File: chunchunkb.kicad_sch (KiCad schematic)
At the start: 124 parts, among them J1 BATT, J2 OLED, SW1 SW_Push, SW10 SW_Push, SW11 SW_Push, SW12 SW_Push, SW13 SW_Push, SW14 SW_Push, SW15 SW_Push, SW16 SW_Push, SW17 SW_Push, SW18 SW_Push, SW19 SW_Push, SW2 SW_Push, SW20 SW_Push, SW21 SW_Push, SW22 SW_Push, SW23 SW_Push, SW24 SW_Push, SW25 SW_Push, SW26 SW_Push, SW27 SW_Push, SW28 SW_Push, SW29 SW_Push, SW3 SW_Push, SW30 SW_Push, SW31 EC11, SW32 SW_Push, SW33 SW_Push, SW34 SW_Push, SW35 SW_Push, SW36 SW_Push, SW4 SW_Push, SW5 SW_Push, SW6 SW_Push, SW7 SW_Push, SW8 SW_Push, SW9 SW_Push

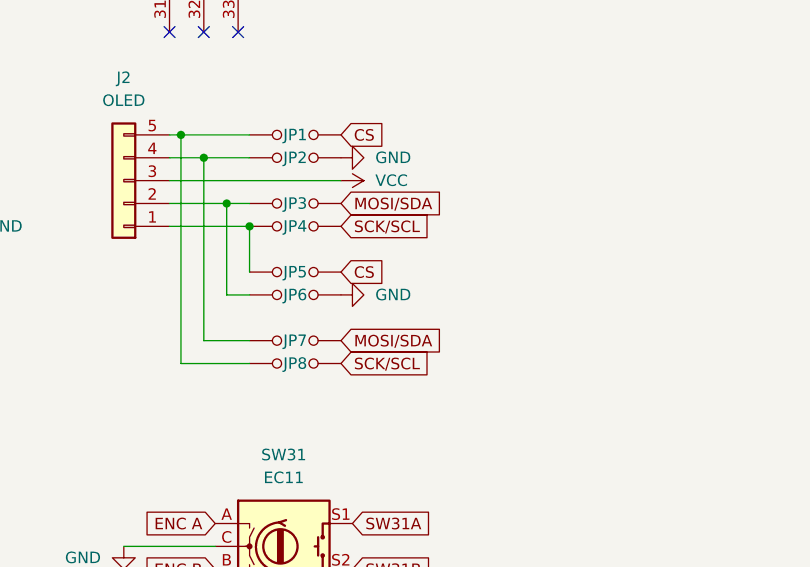
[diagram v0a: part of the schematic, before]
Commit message: snapshot
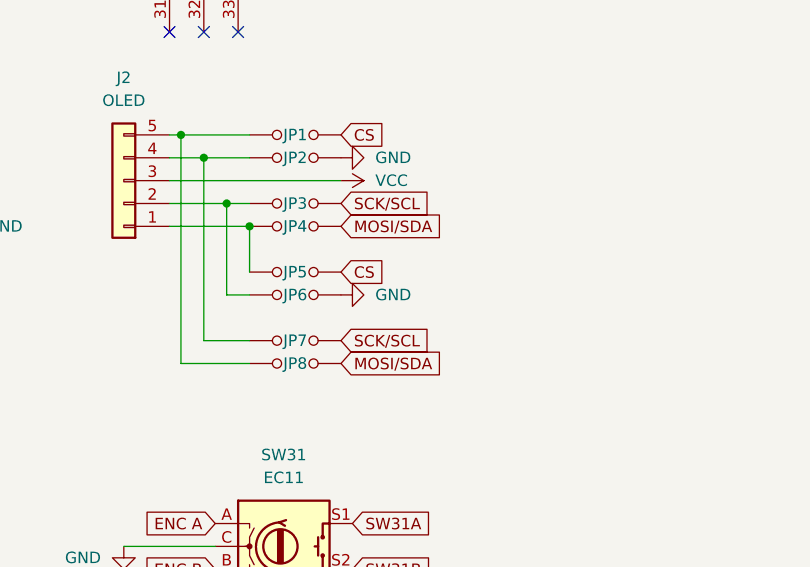
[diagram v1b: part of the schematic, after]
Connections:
- net MOSI/SDA: now also JP4.2 (B), JP8.2 (B); no longer JP3.2 (B), JP7.2 (B)
- net SCK/SCL: now also JP3.2 (B), JP7.2 (B); no longer JP4.2 (B), JP8.2 (B)

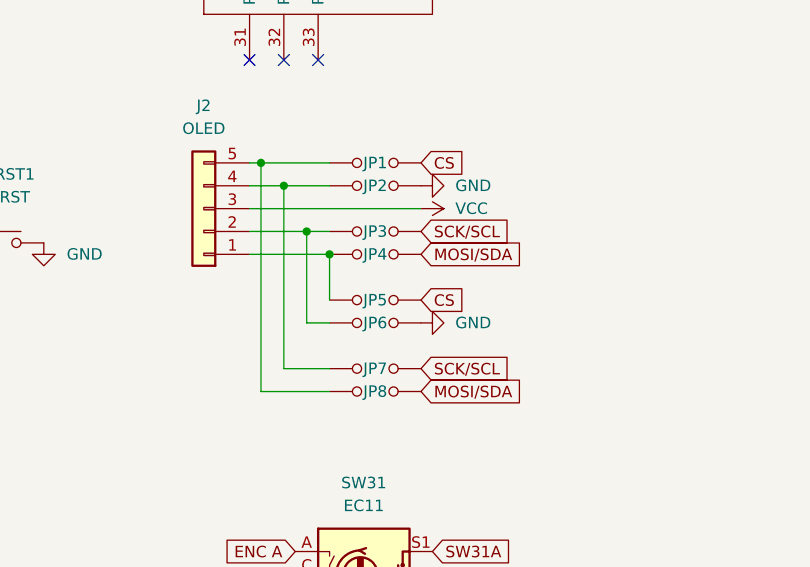
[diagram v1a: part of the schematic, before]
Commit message: snapshot
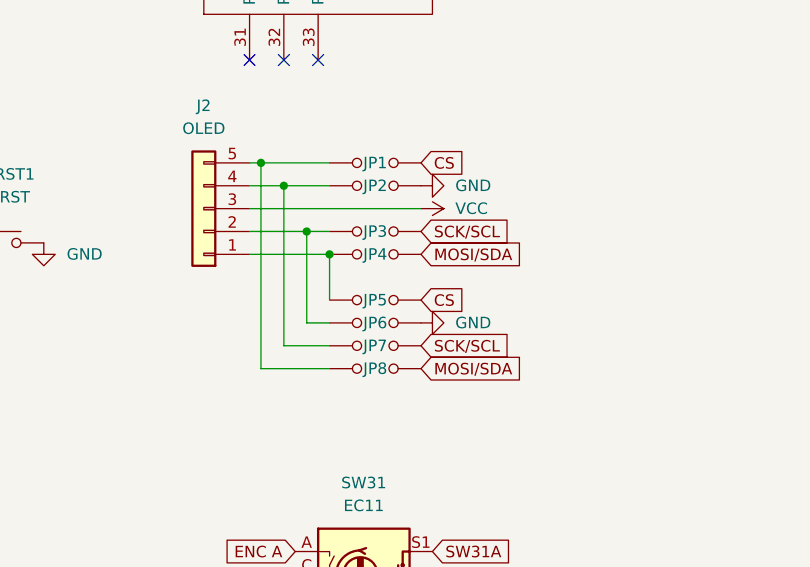
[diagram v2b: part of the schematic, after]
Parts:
- D1, D10, D11, D12, D13, D14, D15, D16, D17, D18, D19, D2, D20, D21, D22, D23, D24, D25, D26, D27, D28, D29, D3, D30, D31, D32, D33, D34, D35, D36, D4, D5, D6, D7, D8, D9: footprint chunchunkb:D_SOD-123 -> chunchunkb:crkbd-diode
- U1: footprint chunchunkb:ProMicro_R2 -> chunchunkb:ProMicro DUAL
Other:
- moved on the sheet: JP7, JP8
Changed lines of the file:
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@@
 	(wire
 		(pts
-			(xy 77.47 113.03) (xy 72.39 113.03)
+			(xy 77.47 110.49) (xy 72.39 110.49)
 		)
 		(stroke
@@
 	(wire
 		(pts
-			(xy 77.47 115.57) (xy 69.85 115.57)
+			(xy 77.47 113.03) (xy 69.85 113.03)
 		)
 		(stroke
@@
 	(wire
 		(pts
-			(xy 69.85 115.57) (xy 69.85 90.17)
+			(xy 69.85 113.03) (xy 69.85 90.17)
 		)
 		(stroke
@@
 	(wire
 		(pts
-			(xy 72.39 113.03) (xy 72.39 92.71)
+			(xy 72.39 110.49) (xy 72.39 92.71)
 		)
 		(stroke
@@
 	(global_label "SCK{slash}SCL"
 		(shape input)
-		(at 87.63 113.03 0)
+		(at 87.63 110.49 0)
 		(fields_autoplaced yes)
 		(effects
@@
 		)
 		(property "Intersheetrefs" "${INTERSHEET_REFS}"
-			(at 97.8534 113.03 0)
+			(at 97.8534 110.49 0)
 			(hide yes)
 			(show_name no)
@@
 	(global_label "MOSI{slash}SDA"
 		(shape input)
-		(at 87.63 115.57 0)
+		(at 87.63 113.03 0)
 		(fields_autoplaced yes)
 		(effects
@@
 		)
 		(property "Intersheetrefs" "${INTERSHEET_REFS}"
-			(at 98.9192 115.57 0)
+			(at 98.9192 113.03 0)
 			(hide yes)
 			(show_name no)
@@
 			)
 		)
-		(property "Footprint" "chunchunkb:D_SOD-123"
+		(property "Footprint" "chunchunkb:crkbd-diode"
 			(at 175.895 83.82 0)
 			(hide yes)
@@
 			)
 		)
-		(property "Footprint" "chunchunkb:D_SOD-123"
+		(property "Footprint" "chunchunkb:crkbd-diode"
 			(at 161.925 119.38 0)
 			(hide yes)
@@
 			)
 		)
-		(property "Footprint" "chunchunkb:D_SOD-123"
+		(property "Footprint" "chunchunkb:crkbd-diode"
 			(at 203.835 66.04 0)
 			(hide yes)
@@
 			)
 		)
-		(property "Footprint" "chunchunkb:D_SOD-123"
+		(property "Footprint" "chunchunkb:crkbd-diode"
 			(at 189.865 119.38 0)
 			(hide yes)
@@
 			)
 		)
-		(property "Footprint" "chunchunkb:D_SOD-123"
+		(property "Footprint" "chunchunkb:crkbd-diode"
 			(at 175.895 66.04 0)
 			(hide yes)
@@
 	(symbol
 		(lib_id "chunchunkb:jumper")
-		(at 82.55 115.57 0)
+		(at 82.55 113.03 0)
 		(unit 1)
 		(body_style 1)
@@
 		(fields_autoplaced yes)
 		(property "Reference" "JP8"
-			(at 82.55 115.57 0)
+			(at 82.55 113.03 0)
 			(show_name no)
 			(do_not_autoplace yes)
@@
 		)
 		(property "Value" "jumper"
-			(at 82.55 117.856 0)
+			(at 82.55 115.316 0)
 			(hide yes)
 			(show_name no)
@@
 		)
 		(property "Footprint" "chunchunkb:Jumper"
-			(at 82.55 115.57 0)
+			(at 82.55 113.03 0)
 			(hide yes)
 			(show_name no)
@@
 		)
 		(property "Datasheet" ""
-			(at 82.55 115.57 0)
+			(at 82.55 113.03 0)
 			(hide yes)
 			(show_name no)
@@
 		)
 		(property "Description" "Jumper, 2-pole, open"
-			(at 82.55 115.57 0)
+			(at 82.55 113.03 0)
 			(hide yes)
 			(show_name no)
@@
 			)
 		)
-		(property "Footprint" "chunchunkb:D_SOD-123"
+		(property "Footprint" "chunchunkb:crkbd-diode"
 			(at 217.805 83.82 0)
 			(hide yes)
@@
 			)
 		)
-		(property "Footprint" "chunchunkb:D_SOD-123"
+		(property "Footprint" "chunchunkb:crkbd-diode"
 			(at 231.775 48.26 0)
 			(hide yes)
@@
 			)
 		)
-		(property "Footprint" "chunchunkb:D_SOD-123"
+		(property "Footprint" "chunchunkb:crkbd-diode"
 			(at 203.835 83.82 0)
 			(hide yes)
@@
 			)
 		)
-		(property "Footprint" "chunchunkb:D_SOD-123"
+		(property "Footprint" "chunchunkb:crkbd-diode"
 			(at 175.895 119.38 0)
 			(hide yes)
@@
 			)
 		)
-		(property "Footprint" "chunchunkb:D_SOD-123"
+		(property "Footprint" "chunchunkb:crkbd-diode"
 			(at 231.775 101.6 0)
 			(hide yes)
@@
 			)
 		)
-		(property "Footprint" "chunchunkb:D_SOD-123"
+		(property "Footprint" "chunchunkb:crkbd-diode"
 			(at 217.805 137.16 0)
 			(hide yes)
@@
 			)
 		)
-		(property "Footprint" "chunchunkb:D_SOD-123"
+		(property "Footprint" "chunchunkb:crkbd-diode"
 			(at 231.775 66.04 0)
 			(hide yes)
@@
 			)
 		)
-		(property "Footprint" "chunchunkb:D_SOD-123"
+		(property "Footprint" "chunchunkb:crkbd-diode"
 			(at 217.805 48.26 0)
 			(hide yes)
@@
 			)
 		)
-		(property "Footprint" "chunchunkb:D_SOD-123"
+		(property "Footprint" "chunchunkb:crkbd-diode"
 			(at 161.925 101.6 0)
 			(hide yes)
@@
 			)
 		)
-		(property "Footprint" "chunchunkb:D_SOD-123"
+		(property "Footprint" "chunchunkb:crkbd-diode"
 			(at 189.865 101.6 0)
 			(hide yes)
@@
 			)
 		)
-		(property "Footprint" "chunchunkb:D_SOD-123"
+		(property "Footprint" "chunchunkb:crkbd-diode"
 			(at 161.925 83.82 0)
 			(hide yes)
@@
 			)
 		)
-		(property "Footprint" "chunchunkb:D_SOD-123"
+		(property "Footprint" "chunchunkb:crkbd-diode"
 			(at 203.835 119.38 0)
 			(hide yes)
@@
 			)
 		)
-		(property "Footprint" "chunchunkb:D_SOD-123"
+		(property "Footprint" "chunchunkb:crkbd-diode"
 			(at 217.805 101.6 0)
 			(hide yes)
@@
 			)
 		)
-		(property "Footprint" "chunchunkb:D_SOD-123"
+		(property "Footprint" "chunchunkb:crkbd-diode"
 			(at 175.895 101.6 0)
 			(hide yes)
@@
 			)
 		)
-		(property "Footprint" "chunchunkb:D_SOD-123"
+		(property "Footprint" "chunchunkb:crkbd-diode"
 			(at 189.865 137.16 0)
 			(hide yes)
@@
 			)
 		)
-		(property "Footprint" "chunchunkb:D_SOD-123"
+		(property "Footprint" "chunchunkb:crkbd-diode"
 			(at 217.805 66.04 0)
 			(hide yes)
@@
 			)
 		)
-		(property "Footprint" "chunchunkb:D_SOD-123"
+		(property "Footprint" "chunchunkb:crkbd-diode"
 			(at 161.925 137.16 0)
 			(hide yes)
@@
 			)
 		)
-		(property "Footprint" "chunchunkb:D_SOD-123"
+		(property "Footprint" "chunchunkb:crkbd-diode"
 			(at 189.865 83.82 0)
 			(hide yes)
@@
 	(symbol
 		(lib_id "chunchunkb:jumper")
-		(at 82.55 113.03 0)
+		(at 82.55 110.49 0)
 		(unit 1)
 		(body_style 1)
@@
 		(fields_autoplaced yes)
 		(property "Reference" "JP7"
-			(at 82.55 113.03 0)
+			(at 82.55 110.49 0)
 			(show_name no)
 			(do_not_autoplace yes)
@@
 		)
 		(property "Value" "jumper"
-			(at 82.55 115.316 0)
+			(at 82.55 112.776 0)
 			(hide yes)
 			(show_name no)
@@
 		)
 		(property "Footprint" "chunchunkb:Jumper"
-			(at 82.55 113.03 0)
+			(at 82.55 110.49 0)
 			(hide yes)
 			(show_name no)
@@
 		)
 		(property "Datasheet" ""
-			(at 82.55 113.03 0)
+			(at 82.55 110.49 0)
 			(hide yes)
 			(show_name no)
@@
 		)
 		(property "Description" "Jumper, 2-pole, open"
-			(at 82.55 113.03 0)
+			(at 82.55 110.49 0)
 			(hide yes)
 			(show_name no)
@@
 			)
 		)
-		(property "Footprint" "chunchunkb:D_SOD-123"
+		(property "Footprint" "chunchunkb:crkbd-diode"
 			(at 189.865 66.04 0)
 			(hide yes)
@@
 			)
 		)
-		(property "Footprint" "chunchunkb:ProMicro_R2"
+		(property "Footprint" "chunchunkb:ProMicro DUAL"
 			(at 102.87 115.57 90)
 			(hide yes)
@@
 			)
 		)
-		(property "Footprint" "chunchunkb:D_SOD-123"
+		(property "Footprint" "chunchunkb:crkbd-diode"
 			(at 231.775 83.82 0)
 			(hide yes)
@@
 			)
 		)
-		(property "Footprint" "chunchunkb:D_SOD-123"
+		(property "Footprint" "chunchunkb:crkbd-diode"
 			(at 203.835 101.6 0)
 			(hide yes)
@@
 			)
 		)
-		(property "Footprint" "chunchunkb:D_SOD-123"
+		(property "Footprint" "chunchunkb:crkbd-diode"
 			(at 161.925 48.26 0)
 			(hide yes)
@@
 			)
 		)
-		(property "Footprint" "chunchunkb:D_SOD-123"
+		(property "Footprint" "chunchunkb:crkbd-diode"
 			(at 161.925 66.04 0)
 			(hide yes)
@@
 			)
 		)
-		(property "Footprint" "chunchunkb:D_SOD-123"
+		(property "Footprint" "chunchunkb:crkbd-diode"
 			(at 231.775 119.38 0)
 			(hide yes)
@@
 			)
 		)
-		(property "Footprint" "chunchunkb:D_SOD-123"
+		(property "Footprint" "chunchunkb:crkbd-diode"
 			(at 189.865 48.26 0)
 			(hide yes)
@@
 			)
 		)
-		(property "Footprint" "chunchunkb:D_SOD-123"
+		(property "Footprint" "chunchunkb:crkbd-diode"
 			(at 203.835 48.26 0)
 			(hide yes)
@@
 			)
 		)
-		(property "Footprint" "chunchunkb:D_SOD-123"
+		(property "Footprint" "chunchunkb:crkbd-diode"
 			(at 217.805 119.38 0)
 			(hide yes)
@@
 			)
 		)
-		(property "Footprint" "chunchunkb:D_SOD-123"
+		(property "Footprint" "chunchunkb:crkbd-diode"
 			(at 231.775 137.16 0)
 			(hide yes)
@@
 			)
 		)
-		(property "Footprint" "chunchunkb:D_SOD-123"
+		(property "Footprint" "chunchunkb:crkbd-diode"
 			(at 203.835 137.16 0)
 			(hide yes)
@@
 			)
 		)
-		(property "Footprint" "chunchunkb:D_SOD-123"
+		(property "Footprint" "chunchunkb:crkbd-diode"
 			(at 175.895 137.16 0)
 			(hide yes)
@@
 			)
 		)
-		(property "Footprint" "chunchunkb:D_SOD-123"
+		(property "Footprint" "chunchunkb:crkbd-diode"
 			(at 175.895 48.26 0)
 			(hide yes)
